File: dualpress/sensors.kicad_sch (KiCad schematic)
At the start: 5 parts, among them J1 WATCH_RELAIS, U3 PC817

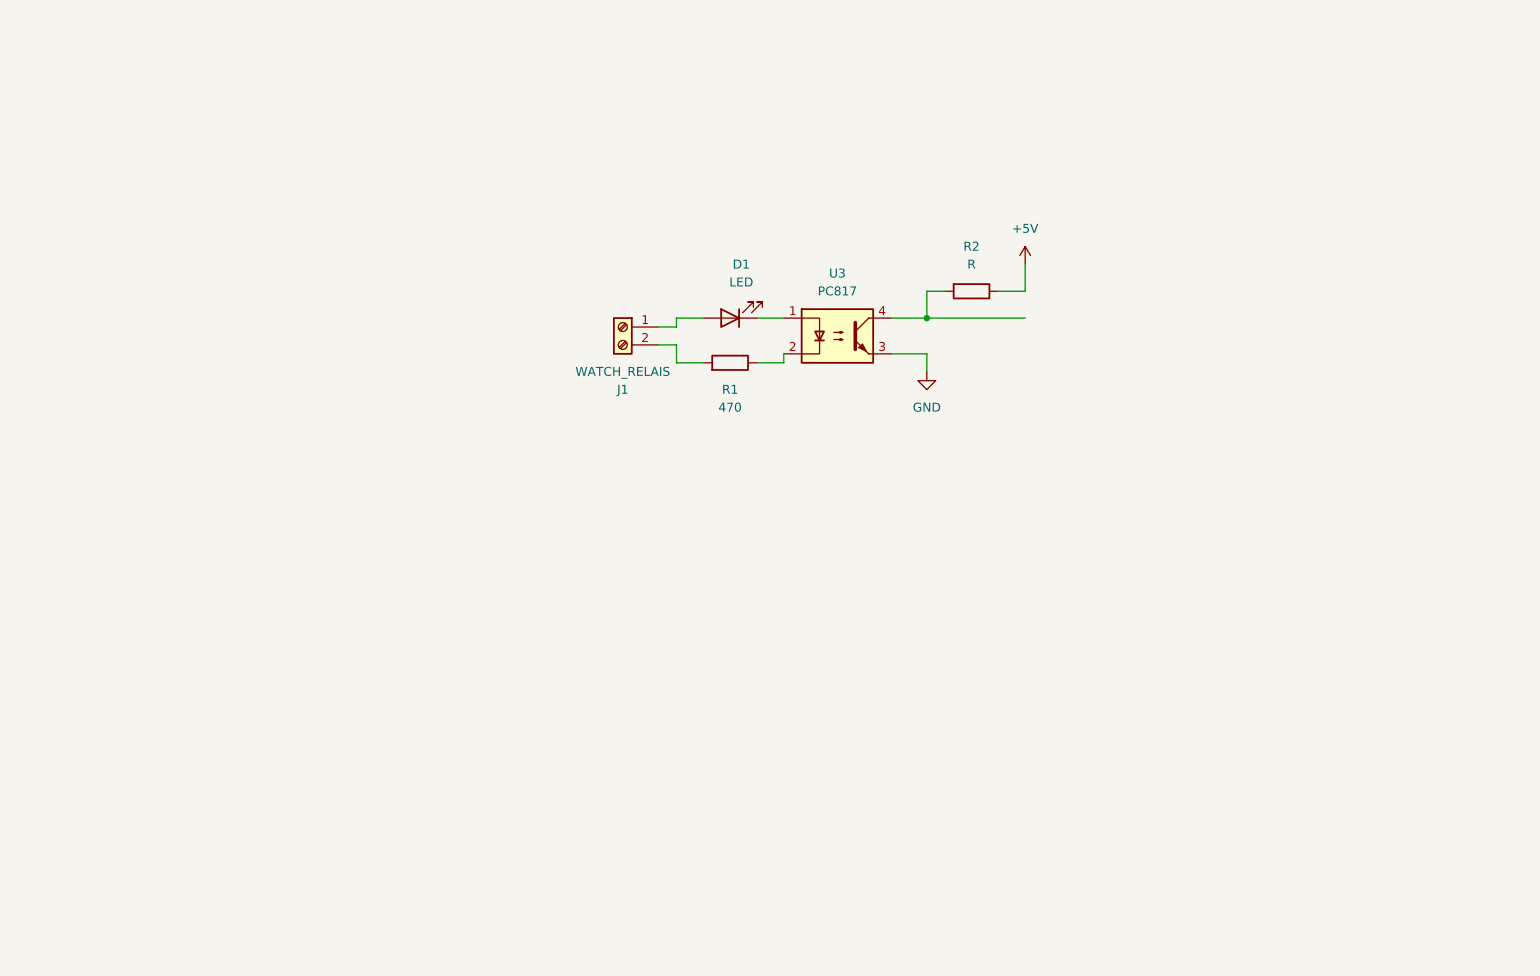
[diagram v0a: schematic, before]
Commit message: schematic done
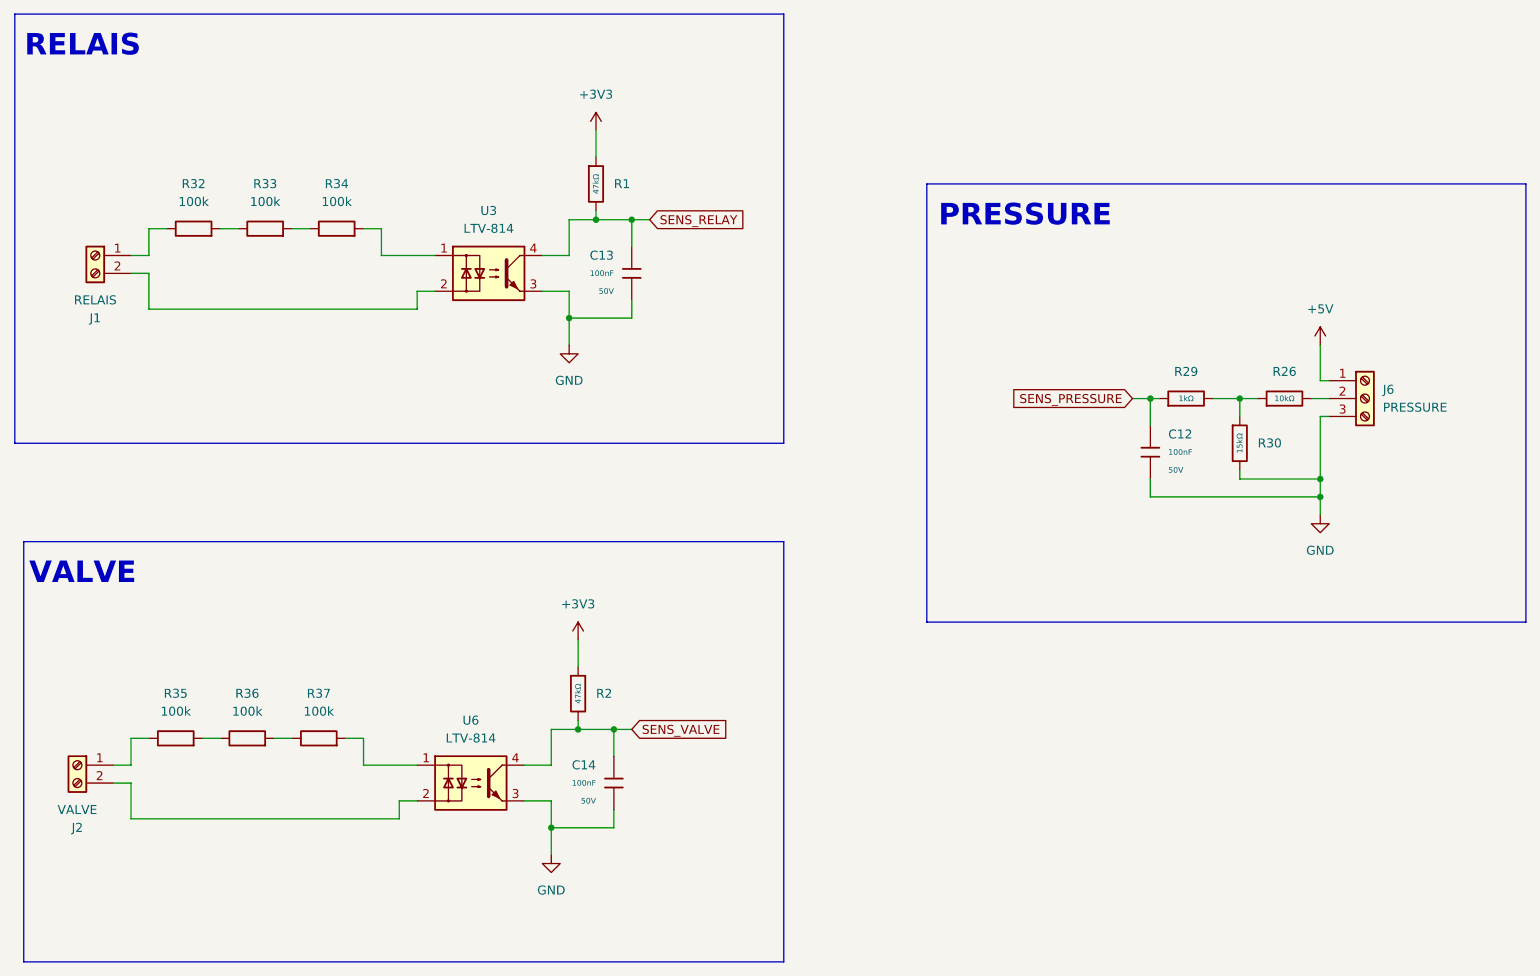
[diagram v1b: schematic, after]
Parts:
- removed D1: LED, Diode_SMD:D_0201_0603Metric, symbol Device:LED
- removed R1: 470, Resistor_SMD:R_0805_2012Metric, symbol Device:R
- removed R2: R, symbol Device:R
- removed U3: PC817, Package_DIP:DIP-4_W7.62mm, symbol Isolator:PC817
- added C12, C13, C14: 100nF, PCM_JLCPCB:C_0603, symbol PCM_JLCPCB-Capacitors:0603,100nF
- added J2: VALVE, Connector_JST:JST_XH_B2B-XH-AM_1x02_P2.50mm_Vertical, symbol Connector:Screw_Terminal_01x02
- added J6: PRESSURE, symbol Connector:Screw_Terminal_01x03
- added R1, R2: 47kΩ, PCM_JLCPCB:R_0603, symbol PCM_JLCPCB-Resistors:0603,47kΩ
- added R26: 10kΩ, PCM_JLCPCB:R_0603, symbol PCM_JLCPCB-Resistors:0603,10kΩ
- added R29: 1kΩ, PCM_JLCPCB:R_0603, symbol PCM_JLCPCB-Resistors:0603,1kΩ
- added R30: 15kΩ, PCM_JLCPCB:R_0603, symbol PCM_JLCPCB-Resistors:0603,15kΩ
- added R32, R33, R34, R35, R36, R37: 100k, Plugin,D4.5xL11.5mm, symbol Device:R
- added U3, U6: LTV-814, Package_DIP:DIP-4_W7.62mm, symbol Isolator:LTV-814
- J1: value WATCH_RELAIS -> RELAIS
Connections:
- net +5V: now also J6.1 (Pin_1)
- net GND: now also C12.2, C13.2, C14.2, J6.3 (Pin_3), R30.2, U3.3, U6.3
- net at J1.1 (Pin_1): now also R32.1
- net at J1.2 (Pin_2): now also U3.2
- new net: R26.1, R29.2, R30.1
- new net: J6.2 (Pin_2), R26.2
- new net: R35.2, R36.1
- new net: R36.2, R37.1
- new net: J2.1 (Pin_1), R35.1
- new net: R34.2, U3.1
- new net: R37.2, U6.1
- new net: J2.2 (Pin_2), U6.2
- new net: R32.2, R33.1
- new net: R33.2, R34.1
- new net +3V3: R1.1, R2.1
- new net SENS_PRESSURE: C12.1, R29.1
- new net SENS_RELAY: C13.1, R1.2, U3.4
- new net SENS_VALVE: C14.1, R2.2, U6.4
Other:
- note added: "PRESSURE"
- note added: "RELAIS"
- note added: "VALVE"
- moved on the sheet: J1
